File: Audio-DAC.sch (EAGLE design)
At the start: 211 parts, among them CON1 USB-5075BR-04-WH, CON2 VOL_CON, CON3 SWD_CON, IC1 3.3V 200mA, IC10 15V, IC11 -15V, IC12 3.3V, IC13 LPC1114FDH28, IC14 7812, IC15 5V, IC16 5V, IC17 3.3V, IC18 TC7WH74FU, IC19 AK4495EQ, IC2 AT32UC3A3256, IC20 TC7WU04FU, IC21 9V, IC22 -9V, IC23 OP275, IC3 OCT_BUFFER-SO6, IC4 OCT_BUFFER-SO6, IC5 OCT_BUFFER-SO6, IC6 OCT_BUFFER-SO6, IC7 OCT_BUFFER-SO6, IC8 OCT_BUFFER-SO6, IC9 7805, Q1 NPN2SC3422, Q2 PNP2SA1359, Q3 NPN2SC3422, Q4 PNP2SA1359, Q5 NPN2SC3325, Q6 NPN2SC3325, SW1 EA2, SW2 EA2, X1 12MHz, X2 22.5792MHz, X3 24.576MHz

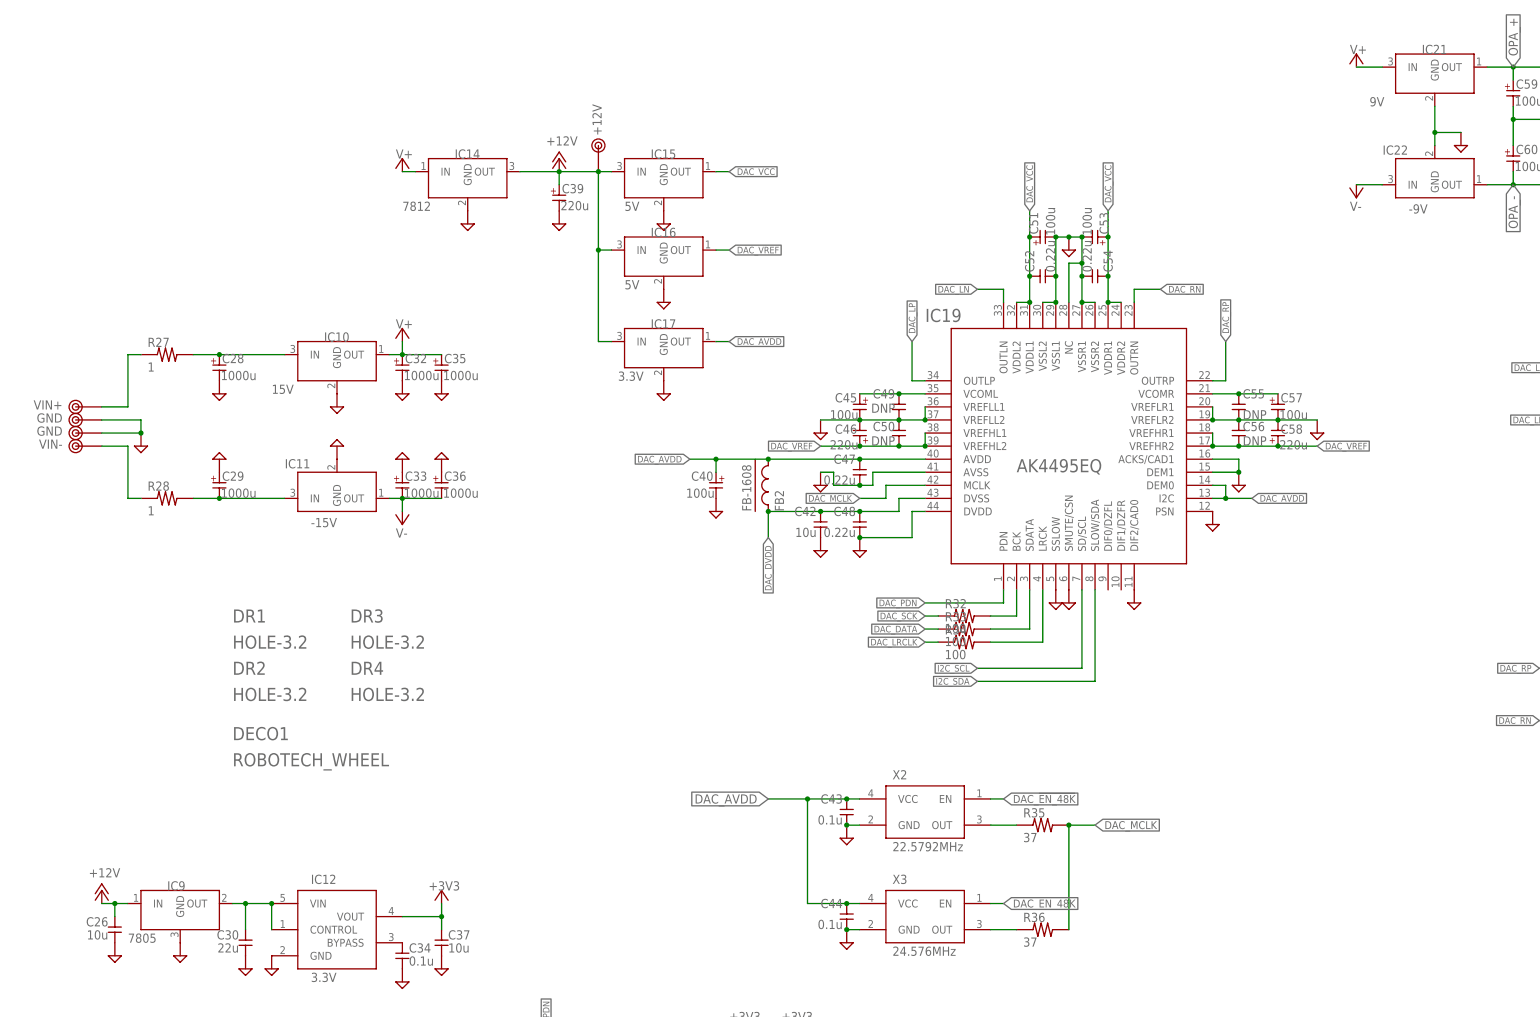
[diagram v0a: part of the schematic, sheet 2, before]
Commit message: 微修正
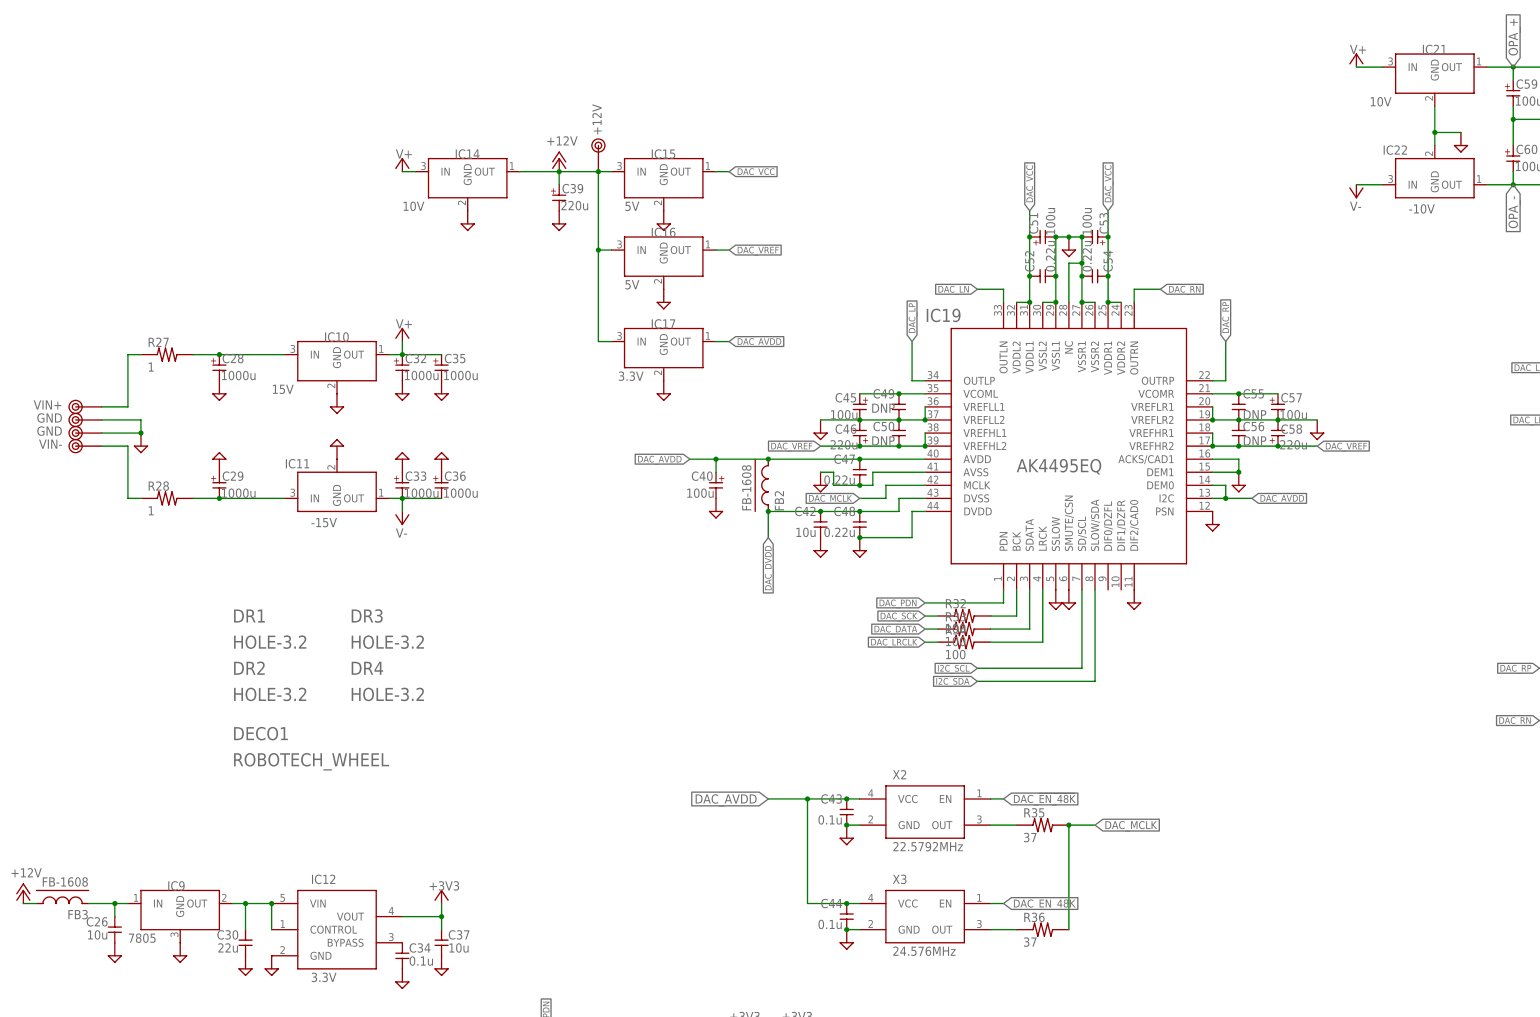
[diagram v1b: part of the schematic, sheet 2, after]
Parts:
- added FB3: FB-1608, my_rcl:FB-1608
- IC14: value 7812 -> 10V; device my_ic:78X-1 -> my_ic:78X-LED
- IC21: value 9V -> 10V
- IC22: value -9V -> -10V
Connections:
- new net N$56: C26.1, FB3.2, IC9.IN
- net +12V: now also FB3.1; no longer C26.1, IC9.IN
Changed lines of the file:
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@@
 <part name="SUPPLY70" library="my_supply" deviceset="GND" device=""/>
 <part name="SUPPLY71" library="my_supply" deviceset="GND" device=""/>
-<part name="IC14" library="my_ic" deviceset="78X" device="-1" value="7812"/>
+<part name="IC14" library="my_ic" deviceset="78X" device="-LED" value="10V"/>
 <part name="IC15" library="my_ic" deviceset="78X" device="-LED" value="5V"/>
 <part name="IC16" library="my_ic" deviceset="78X" device="-LED" value="5V"/>
@@
 <part name="C60" library="my_rcl" deviceset="CPOL" device="E2.5-8" value="100u"/>
 <part name="SUPPLY82" library="my_supply" deviceset="GND" device=""/>
-<part name="IC21" library="my_ic" deviceset="78X" device="-LED" value="9V"/>
-<part name="IC22" library="my_ic" deviceset="79X" device="-LED" value="-9V"/>
+<part name="IC21" library="my_ic" deviceset="78X" device="-LED" value="10V"/>
+<part name="IC22" library="my_ic" deviceset="79X" device="-LED" value="-10V"/>
 <part name="SUPPLY83" library="my_supply" deviceset="GND" device=""/>
 <part name="C40" library="my_rcl" deviceset="CPOL" device="E2.5-6.5" value="100u"/>
@@
 <part name="R26" library="my_rcl" deviceset="R" device="-1608" value="1.5k"/>
 <part name="SUPPLY132" library="my_supply" deviceset="GND" device=""/>
+<part name="FB3" library="my_rcl" deviceset="FB" device="-1608"/>
 </parts>
 <sheets>
@@
 <attribute name="VALUE" x="45.72" y="-25.4" size="1.778" layer="96"/>
 </instance>
-<instance part="P+3" gate="1" x="-180.34" y="20.32" smashed="yes">
-<attribute name="VALUE" x="-182.88" y="22.86" size="1.778" layer="96"/>
+<instance part="P+3" gate="1" x="-195.58" y="20.32" smashed="yes">
+<attribute name="VALUE" x="-198.12" y="22.86" size="1.778" layer="96"/>
 </instance>
 <instance part="CON3" gate="G$1" x="-55.88" y="-63.5" smashed="yes">
@@
 <attribute name="VALUE" x="-154.94" y="44.45" size="2.54" layer="96"/>
 </instance>
+<instance part="FB3" gate="G$1" x="-187.96" y="17.78" smashed="yes" rot="R90">
+<attribute name="NAME" x="-182.88" y="16.51" size="1.778" layer="95" rot="R180"/>
+<attribute name="VALUE" x="-182.88" y="22.86" size="1.778" layer="96" rot="R180"/>
+</instance>
 </instances>
 <busses>
@@
 </segment>
 <segment>
-<pinref part="IC9" gate="G$1" pin="IN"/>
-<wire x1="-175.26" y1="17.78" x2="-177.8" y2="17.78" width="0.1524" layer="91"/>
-<pinref part="C26" gate="G$1" pin="1"/>
-<wire x1="-177.8" y1="17.78" x2="-180.34" y2="17.78" width="0.1524" layer="91"/>
-<wire x1="-177.8" y1="15.24" x2="-177.8" y2="17.78" width="0.1524" layer="91"/>
-<junction x="-177.8" y="17.78"/>
 <pinref part="P+3" gate="1" pin="+12V"/>
+<wire x1="-193.04" y1="17.78" x2="-195.58" y2="17.78" width="0.1524" layer="91"/>
+<pinref part="FB3" gate="G$1" pin="1"/>
 </segment>
 </net>
@@
 </segment>
 </net>
+<net name="N$56" class="0">
+<segment>
+<pinref part="IC9" gate="G$1" pin="IN"/>
+<wire x1="-175.26" y1="17.78" x2="-177.8" y2="17.78" width="0.1524" layer="91"/>
+<pinref part="C26" gate="G$1" pin="1"/>
+<wire x1="-177.8" y1="15.24" x2="-177.8" y2="17.78" width="0.1524" layer="91"/>
+<junction x="-177.8" y="17.78"/>
+<wire x1="-177.8" y1="17.78" x2="-182.88" y2="17.78" width="0.1524" layer="91"/>
+<pinref part="FB3" gate="G$1" pin="2"/>
+</segment>
+</net>
